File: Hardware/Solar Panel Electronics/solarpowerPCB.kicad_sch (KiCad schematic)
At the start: 45 parts, among them J3 Conn_01x02_Male, J4 Conn_01x06_Male, J5 Conn_01x02_Male, Q1 MMDT2222A, U1 SN65HVD230, U2 ESP32-PICO-D4

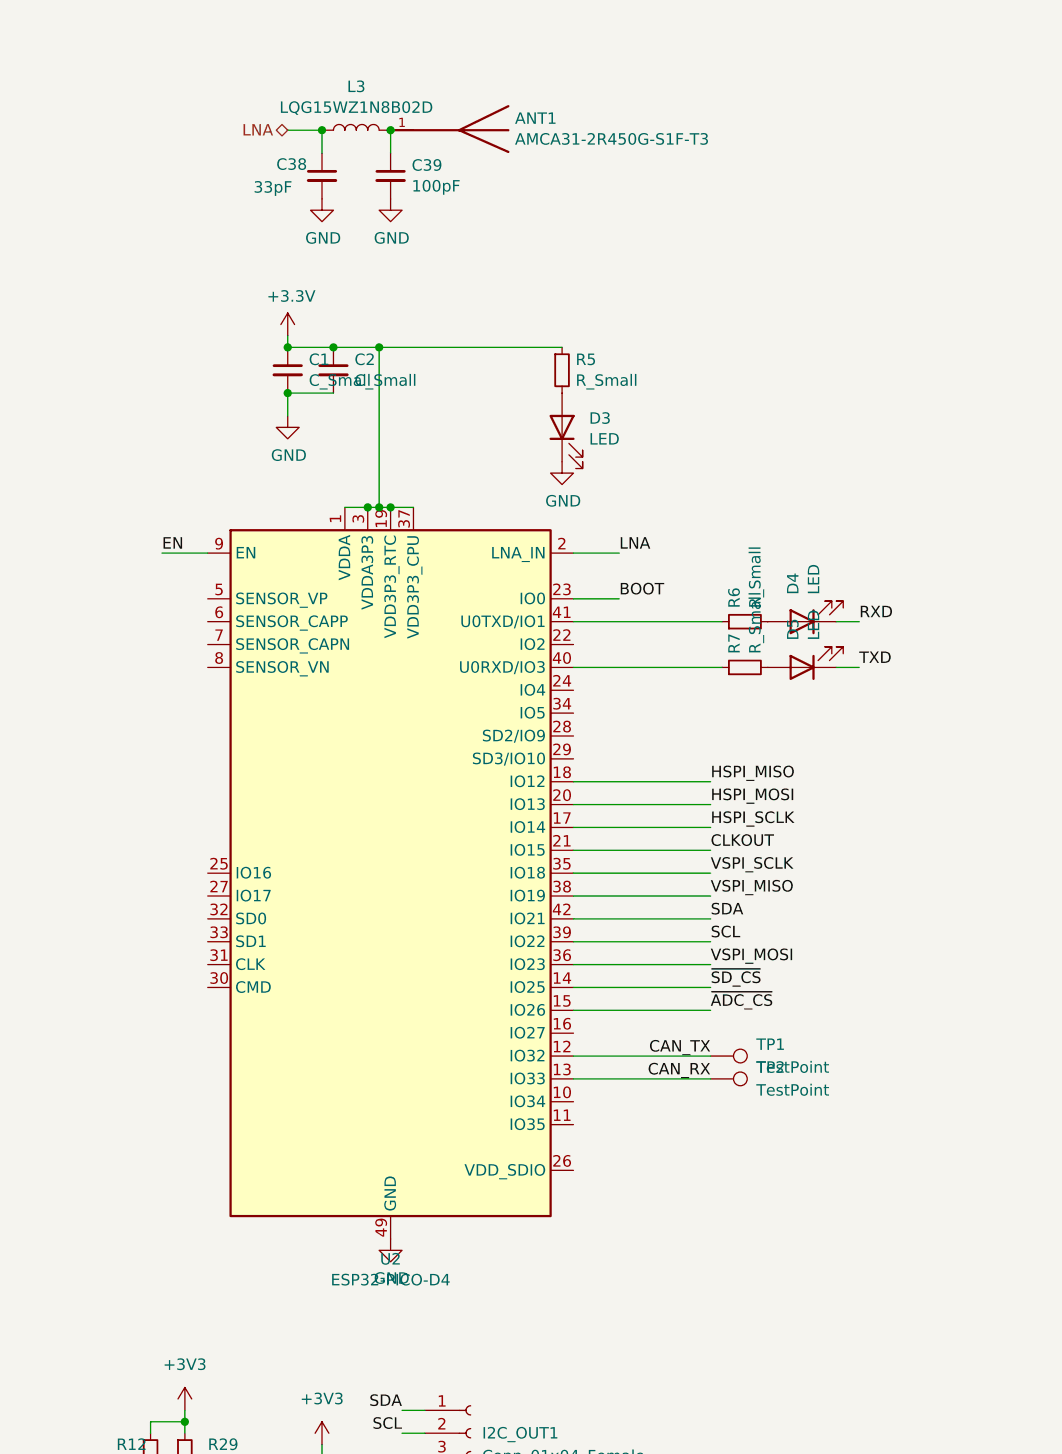
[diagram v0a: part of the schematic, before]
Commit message: Need to do routing.
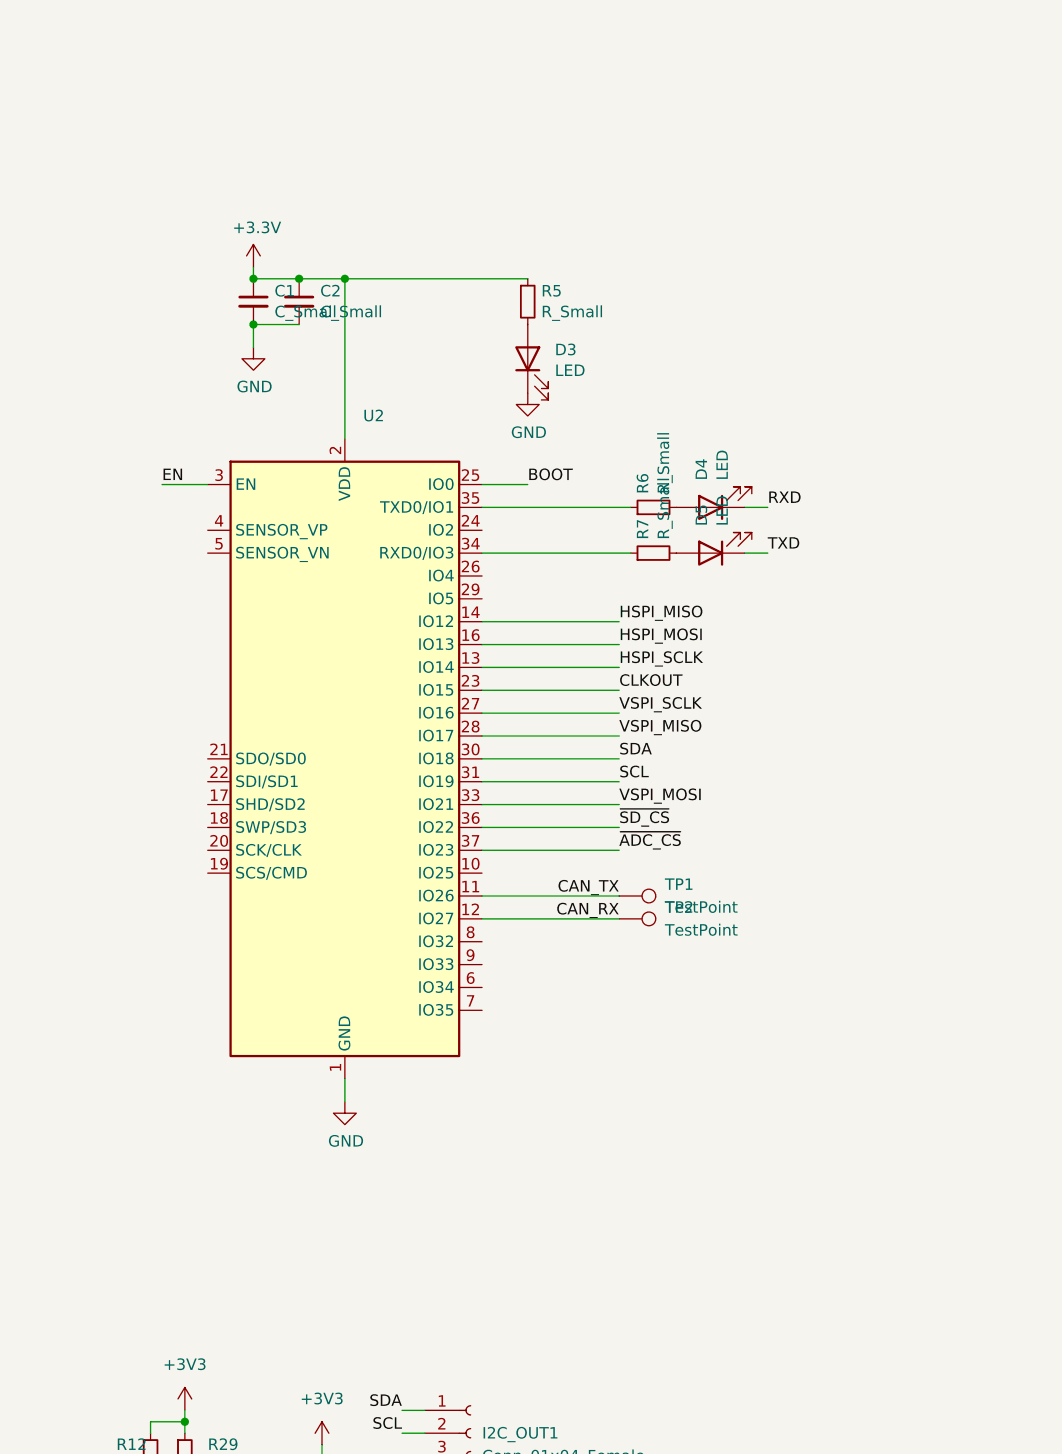
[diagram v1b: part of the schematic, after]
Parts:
- removed ANT1: AMCA31-2R450G-S1F-T3, iclr:ANT_AMCA31-2R450G-S1F-T3, symbol iclr:AMCA31-2R450G-S1F-T3
- removed C38: 33pF, Capacitor_SMD:C_0603_1608Metric, symbol Device:C_Small
- removed C39: 100pF, Capacitor_SMD:C_0603_1608Metric, symbol Device:C_Small
- removed L3: LQG15WZ1N8B02D, Inductor_SMD:L_0603_1608Metric_Pad1.05x0.95mm_HandSolder, symbol Device:L
- removed U2: ESP32-PICO-D4, Package_DFN_QFN:QFN-48-1EP_7x7mm_P0.5mm_EP5.3x5.3mm, symbol RF_Module:ESP32-PICO-D4
- added U2: (no value), symbol RF_Module:ESP32-WROOM-32D
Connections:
- net +3V3: now also U2.2 (VDD)
- net BOOT: now also U2.25 (IO0)
- net CAN_RX: now also U2.12 (IO27)
- net CAN_TX: now also U2.11 (IO26)
- net CLKOUT: now also U2.23 (IO15)
- net EN: now also U2.3 (EN)
- net GND: now also U2.1 (GND), U2.15 (GND), U2.38 (GND), U2.39 (GND)
- net HSPI_MISO: now also U2.14 (IO12)
- net HSPI_MOSI: now also U2.16 (IO13)
- net HSPI_SCLK: now also U2.13 (IO14)
- net SCL: now also U2.31 (IO19)
- net SDA: now also U2.30 (IO18)
- net VSPI_MISO: now also U2.28 (IO17)
- net VSPI_MOSI: now also U2.33 (IO21)
- net VSPI_SCLK: now also U2.27 (IO16)
- net ~{ADC_CS}: now also U2.37 (IO23)
- net ~{SD_CS}: now also U2.36 (IO22)
- net at R6.1: now also U2.35 (TXD0/IO1)
- net at R7.1: now also U2.34 (RXD0/IO3)
